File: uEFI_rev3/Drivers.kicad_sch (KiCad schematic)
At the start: 28 parts, among them Q1 ISL9V5045S3ST, Q2 ISL9V5045S3ST, Q3 ISL9V5045S3ST, Q4 ISL9V5045S3ST

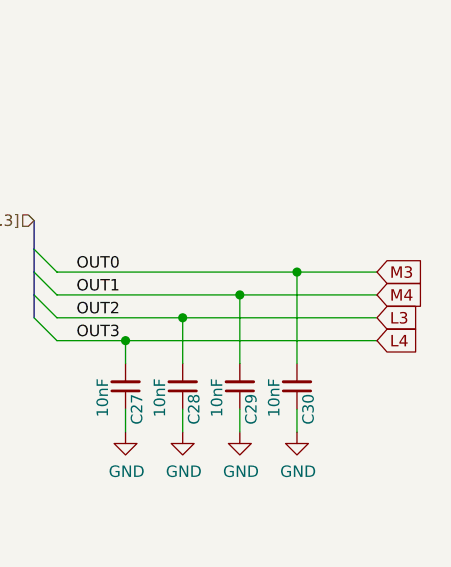
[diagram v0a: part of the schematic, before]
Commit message: rev3, analog inputs
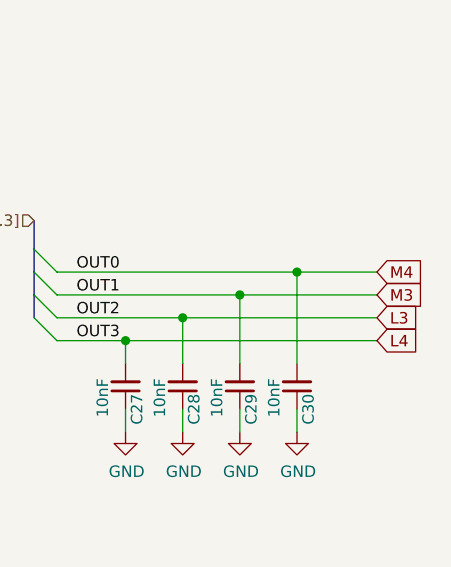
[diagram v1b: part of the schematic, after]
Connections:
- net M3: now also C29.2; no longer C30.2
- net M4: now also C30.2; no longer C29.2
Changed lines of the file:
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@@
     )
   )
-  (global_label "M3" (shape input) (at 165.1 147.32 0)
+  (global_label "M3" (shape input) (at 165.1 149.86 0)
+    (effects (font (size 1.27 1.27)) (justify left))
+    (property "Intersheet References" "${INTERSHEET_REFS}" (id 0) (at 170.1741 149.7806 0)
+      (effects (font (size 1.27 1.27)) (justify left) hide)
+    )
+  )
+  (global_label "M4" (shape input) (at 165.1 147.32 0)
     (effects (font (size 1.27 1.27)) (justify left))
     (property "Intersheet References" "${INTERSHEET_REFS}" (id 0) (at 170.1741 147.2406 0)
       (effects (font (size 1.27 1.27)) (justify left) hide)
     )
-  )
-  (global_label "M4" (shape input) (at 165.1 149.86 0)
-    (effects (font (size 1.27 1.27)) (justify left))
-    (property "Intersheet References" "${INTERSHEET_REFS}" (id 0) (at 170.1741 149.7806 0)
-      (effects (font (size 1.27 1.27)) (justify left) hide)
-    )
